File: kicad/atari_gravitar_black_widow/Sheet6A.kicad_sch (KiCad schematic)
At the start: 10 parts

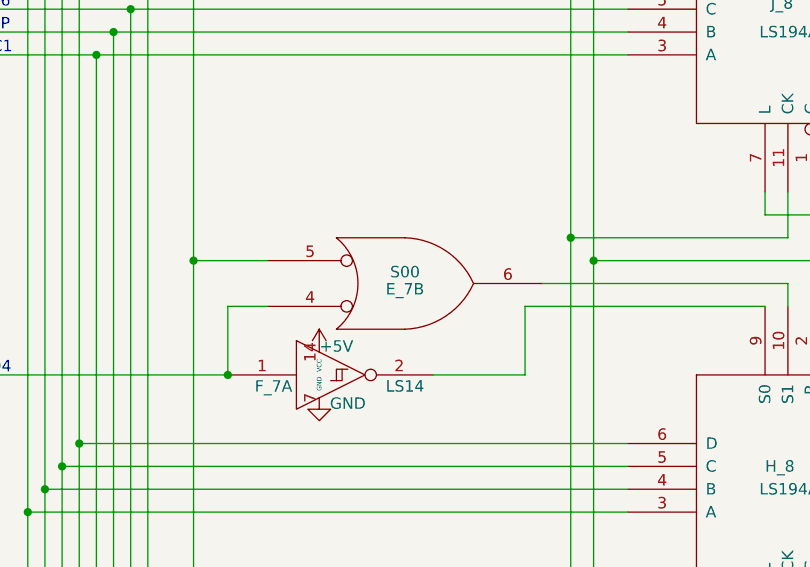
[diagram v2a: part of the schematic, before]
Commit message: Fixed various issues and generated gerber files
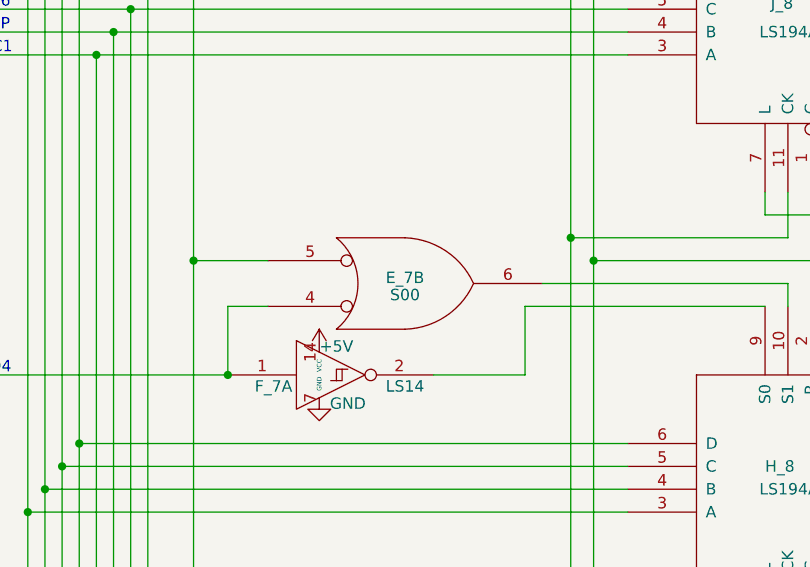
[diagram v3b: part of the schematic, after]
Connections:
- net ~{ENORM}: now also E_7.4; no longer E_7.5
- net ~{LATCH1}: now also E_7.5; no longer E_7.4
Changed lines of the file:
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@@
     (pin "1")
   )
-  (symbol (lib_name "LS00_1") (lib_id "atari_grav_bw:LS00") (at 194.31 157.48 0) (mirror x) (unit 2) (convert 2)
+  (symbol (lib_id "atari_grav_bw:LS00") (at 194.31 157.48 0) (unit 2) (convert 2)
     (in_bom yes) (on_board yes)
-    (property "Reference" "E_7" (id 0) (at 194.31 158.115 0))
-    (property "Value" "S00" (id 1) (at 194.31 156.21 0))
+    (property "Reference" "E_7" (id 0) (at 194.31 156.845 0))
+    (property "Value" "S00" (id 1) (at 194.31 158.75 0))
     (property "Footprint" "Star_Wars_Vector_PCB:DIP14" (id 2) (at 194.31 157.48 0)
       (effects (font (size 1.27 1.27)) hide)
